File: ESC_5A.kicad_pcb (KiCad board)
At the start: 4 copper layers, 0 parts

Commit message: removed two current sense resistors and multiple unsused ADC pins
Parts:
- added C1: .1uF, SamacSys_Parts:CAPC0603X33N, F.Cu at (120.7, 104.8)
- added C10: .1uF, SamacSys_Parts:CAPC2012X110N, F.Cu at (116.7, 108.0)
- added C11: 100uF, SamacSys_Parts:CAPAE660X800N, F.Cu at (71.8, 78.7)
- added C12: 270pF, Capacitor_SMD:C_0402_1005Metric, F.Cu at (116.4, 104.1)
- added C13: .1uF, SamacSys_Parts:CAPC0603X33N, F.Cu at (113.3, 108.0)
- added C2: 10uF, SamacSys_Parts:C1608_Commercial, F.Cu at (118.2, 101.0)
- added C3: 10uF, SamacSys_Parts:CAPC3216X180N, F.Cu at (109.6, 106.0)
- added C4: 1uF, SamacSys_Parts:CAPC1005X55N, F.Cu at (108.5, 108.5)
- added C5: 10uF, SamacSys_Parts:C1608_Commercial, F.Cu at (118.0, 63.1)
- added C6: 10uF, SamacSys_Parts:C1608_Commercial, F.Cu at (125.2, 103.4)
- added C7: 1uF, SamacSys_Parts:CAPC1005X55N, F.Cu at (116.3, 66.2)
- added C8: .1uF, SamacSys_Parts:CAPC0603X33N, F.Cu at (120.7, 106.5)
- added C9: .1uF, SamacSys_Parts:CAPC0603X33N, F.Cu at (123.1, 106.4)
- added D1: WS2812B, LED_SMD:LED_WS2812B_PLCC4_5.0x5.0mm_P3.2mm, F.Cu at (96.2, 75.8)
- added D2: B340AE-13, SamacSys_Parts:DIOM5226X240N, F.Cu at (104.4, 68.3)
- added H1: MountingHole, MountingHole:MountingHole_2.2mm_M2, F.Cu at (111.4, 69.0)
- added H2: MountingHole, MountingHole:MountingHole_2.2mm_M2, F.Cu at (103.4, 73.5)
- added IC1: EEPROM, SamacSys_Parts:SOIC127P600X175-8N, F.Cu at (117.5, 88.3)
- added IC2: 3.3V Reg, SamacSys_Parts:SOIC127P600X170-8N, F.Cu at (112.9, 57.8)
- added IC3: 5V_Reg, SamacSys_Parts:AP1501A50K5G13, F.Cu at (144.1, 78.7)
- added IC4: ATSAMD21E17D-AUT, SamacSys_Parts:QFP80P900X900X120-32N, F.Cu at (103.5, 93.3)
- added J1: USBc, USB4105-GF-A:GCT_USB4105-GF-A, F.Cu at (88.1, 60.6)
- added J2: 5V_PWR, Connector_PinHeader_2.54mm:PinHeader_1x03_P2.54mm_Vertical, F.Cu at (74.2, 56.8)
- added J3: M1, Connector_AMASS:AMASS_XT30U-M_1x02_P5.0mm_Vertical, F.Cu at (84.5, 90.7)
- added J4: M2, Connector_AMASS:AMASS_XT30U-M_1x02_P5.0mm_Vertical, F.Cu at (72.3, 97.9)
- added J5: PWR_IN, Connector_AMASS:AMASS_XT30U-M_1x02_P5.0mm_Vertical, F.Cu at (72.3, 90.7)
- added J6: 5V_PWR, Connector_PinHeader_2.54mm:PinHeader_1x03_P2.54mm_Vertical, F.Cu at (69.6, 56.8)
- added L1: 33uH, SamacSys_Parts:XAL6060333MEC, F.Cu at (71.1, 69.8)
- added R1: 5.1k, Resistor_SMD:R_0402_1005Metric, F.Cu at (93.3, 65.0)
- added R10: 5k, Resistor_SMD:R_0402_1005Metric, F.Cu at (116.3, 110.5)
- added R11: 10k, Resistor_SMD:R_0402_1005Metric, F.Cu at (113.5, 106.1)
- added R12: 10k, Resistor_SMD:R_0402_1005Metric, F.Cu at (119.2, 110.5)
- added R2: 100k, Resistor_SMD:R_0402_1005Metric, F.Cu at (118.5, 55.5)
- added R3: 5.1k, Resistor_SMD:R_0402_1005Metric, F.Cu at (118.5, 57.5)
- added R4: 5.1k, Resistor_SMD:R_0402_1005Metric, F.Cu at (118.5, 59.5)
- added R5: 5.1k, Resistor_SMD:R_0402_1005Metric, F.Cu at (113.4, 110.5)
- added R7: .01, SamacSys_Parts:RESC6430X66N, F.Cu at (73.1, 104.0)
- added R8: 20k, Resistor_SMD:R_0402_1005Metric, F.Cu at (113.5, 104.1)
- added S1: nRST, SamacSys_Parts:LL3301NF065QG, F.Cu at (144.1, 63.5)
- added U1: TB67H420FTG_EL, footprints:TB67H420FTG_EL, F.Cu at (142.9, 97.8)
- added Z1: SZMMSZ4713T1G, SamacSys_Parts:SOD3716X135N, F.Cu at (111.7, 63.2)

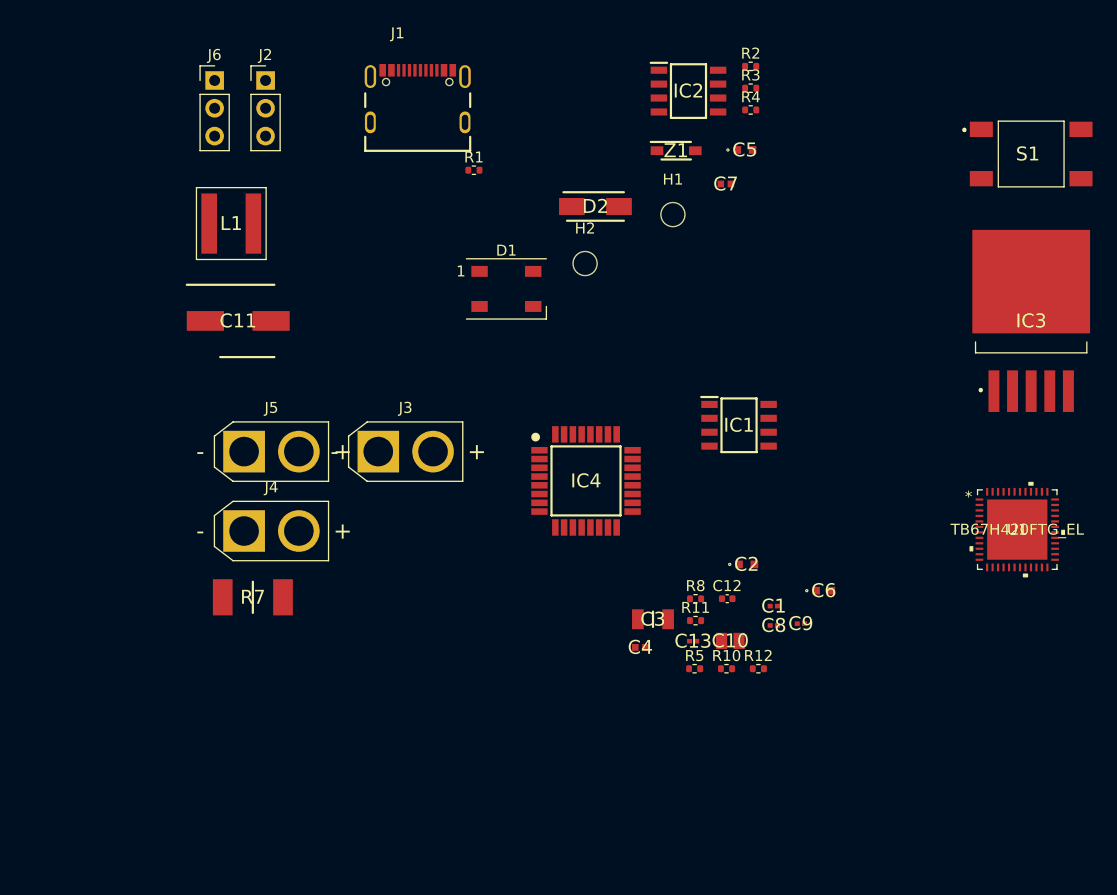
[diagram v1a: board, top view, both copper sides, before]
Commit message: working on layout
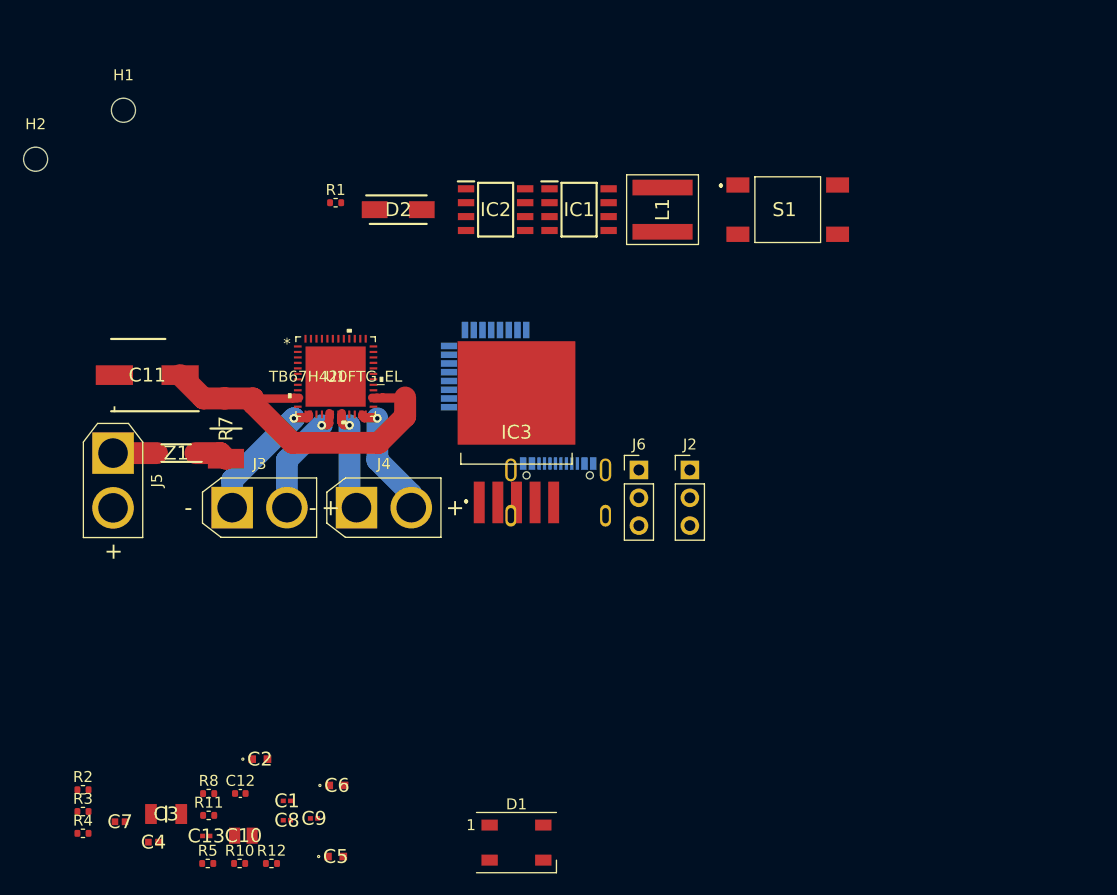
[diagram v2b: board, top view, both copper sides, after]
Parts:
- IC4, J1: moved to B.Cu
- moved R2 89.9 mm to (57.6, 121.5)
- moved R3 89.9 mm to (57.6, 123.5)
- moved R4 89.9 mm to (57.6, 125.5)
- moved C7 80.3 mm to (61.0, 124.5)
- moved C5 74.5 mm to (80.6, 127.6)
- moved U1 63.8 mm to (80.6, 83.8)
- moved Z1 53.3 mm to (66.1, 90.8), turned to 180 degrees
- moved J2 52.6 mm to (113.0, 92.3)
- moved J6 52.6 mm to (108.3, 92.3)
- moved H1 51.1 mm to (61.3, 59.5)
- moved H2 51.1 mm to (53.3, 64.0)
- moved D1 50.6 mm to (97.2, 126.4)
- moved IC3 48.1 mm to (97.2, 88.9)
- moved C1 47.9 mm to (76.2, 122.6)
- moved C10 47.9 mm to (72.2, 125.7)
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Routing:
- net ADC_1: track 0.00 -> 52.7 mm
- net MotorA_Pos: track 0.00 -> 16.8 mm, vias 0 -> 1
- net MotorB_Neg: track 0.00 -> 14.6 mm, vias 0 -> 1
- net MotorA_Neg: track 0.00 -> 13.3 mm, vias 0 -> 1
- net MotorB_Pos: track 0.00 -> 12.6 mm, vias 0 -> 1
- net PWR_IN: track 0.00 -> 4.02 mm
- net ADC_VREFA: track 0.00 -> 3.01 mm
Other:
- copper layers 4 -> 2

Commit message: Working on Layout
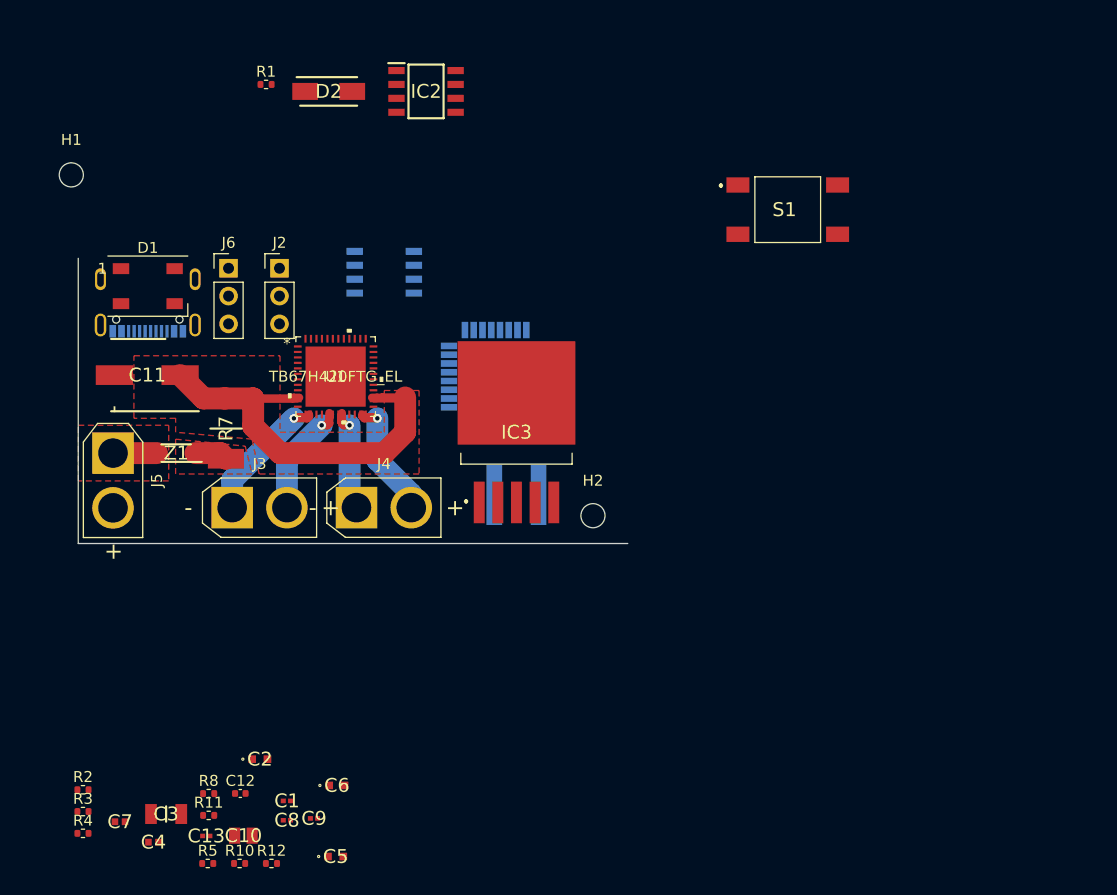
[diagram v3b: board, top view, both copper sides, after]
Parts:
- IC1, L1: moved to B.Cu
- moved D1 60.9 mm to (63.5, 75.6)
- moved H2 60.4 mm to (104.1, 96.5)
- moved J1 43.2 mm to (63.5, 74.9), turned to 0 degrees
- moved J2 41.7 mm to (75.5, 73.9)
- moved J6 41.7 mm to (70.9, 73.9)
- moved L1 29.3 mm to (97.2, 94.6), turned to 0 degrees
- moved IC1 18.7 mm to (85.1, 74.3)
- moved D2 12.5 mm to (80.0, 57.8)
- moved IC2 12.5 mm to (88.9, 57.8)
- moved R1 12.5 mm to (74.3, 57.1)
- moved H1 7.58 mm to (56.5, 65.4)
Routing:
- net ADC_1: track 52.7 -> 56.0 mm
- net MotorA_Pos: track 16.8 -> 15.1 mm
- added copper zone on F.Cu, net ADC_1
- added copper zone on F.Cu, net ADC_VREFA
- added copper zone on F.Cu, net PWR_IN
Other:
- board outline added: 50.2 x 26 mm
